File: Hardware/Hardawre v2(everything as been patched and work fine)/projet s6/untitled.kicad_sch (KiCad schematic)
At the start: 28 parts, among them IC1 QMC5883L, J1 USB_C_Receptacle_USB2.0_14P, J2 OLED, Q1 2N7002K, SW1 Boutton 1, SW2 Boutton 2, U4 USBLC6-2SC6

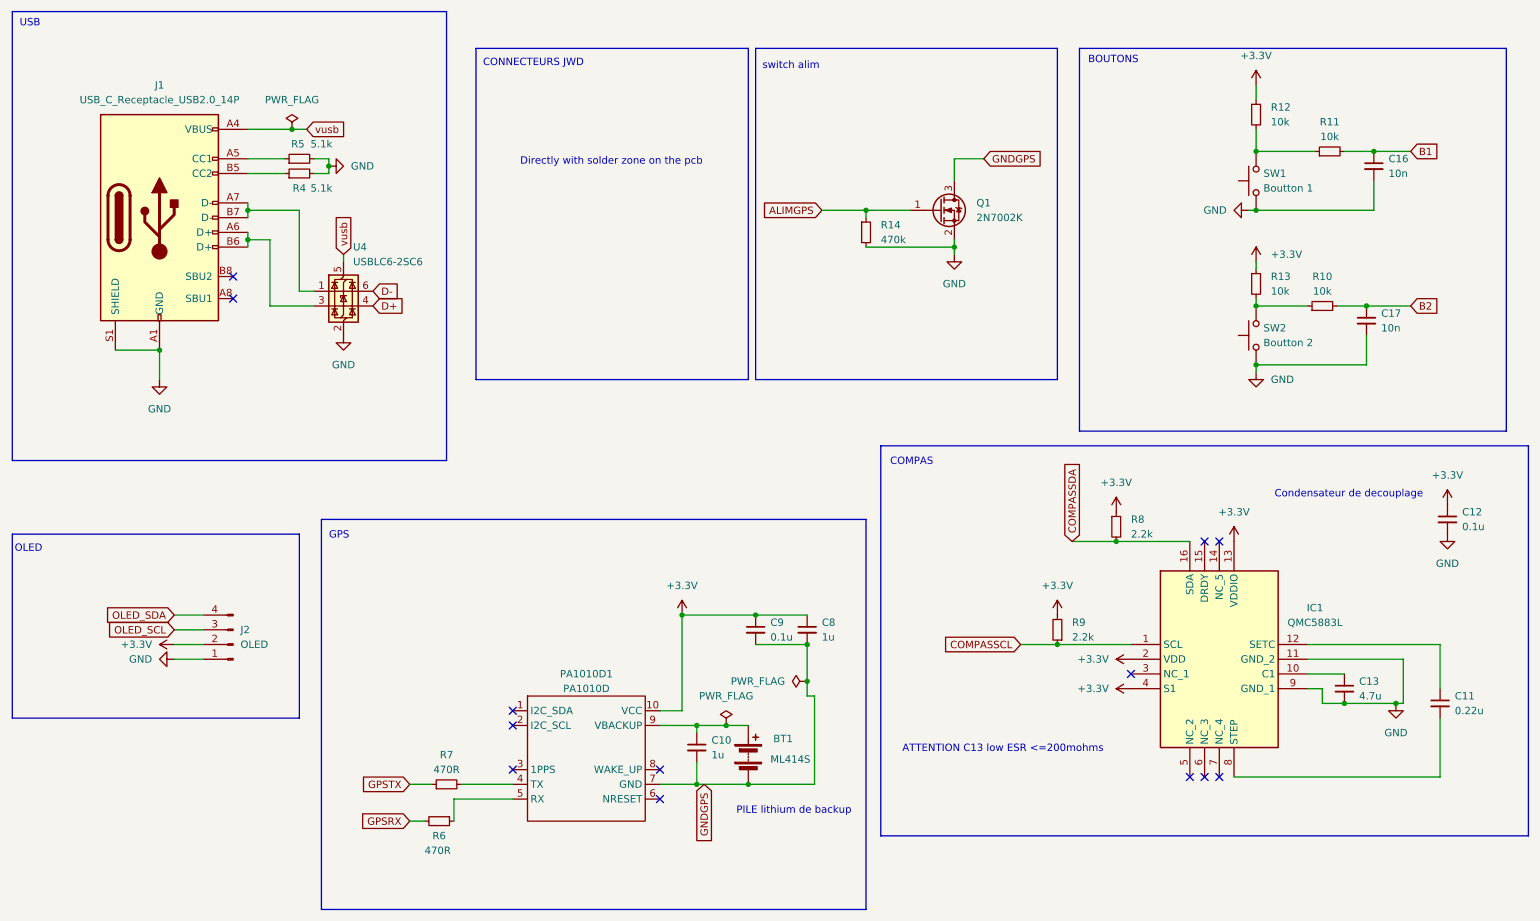
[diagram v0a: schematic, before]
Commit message: gr
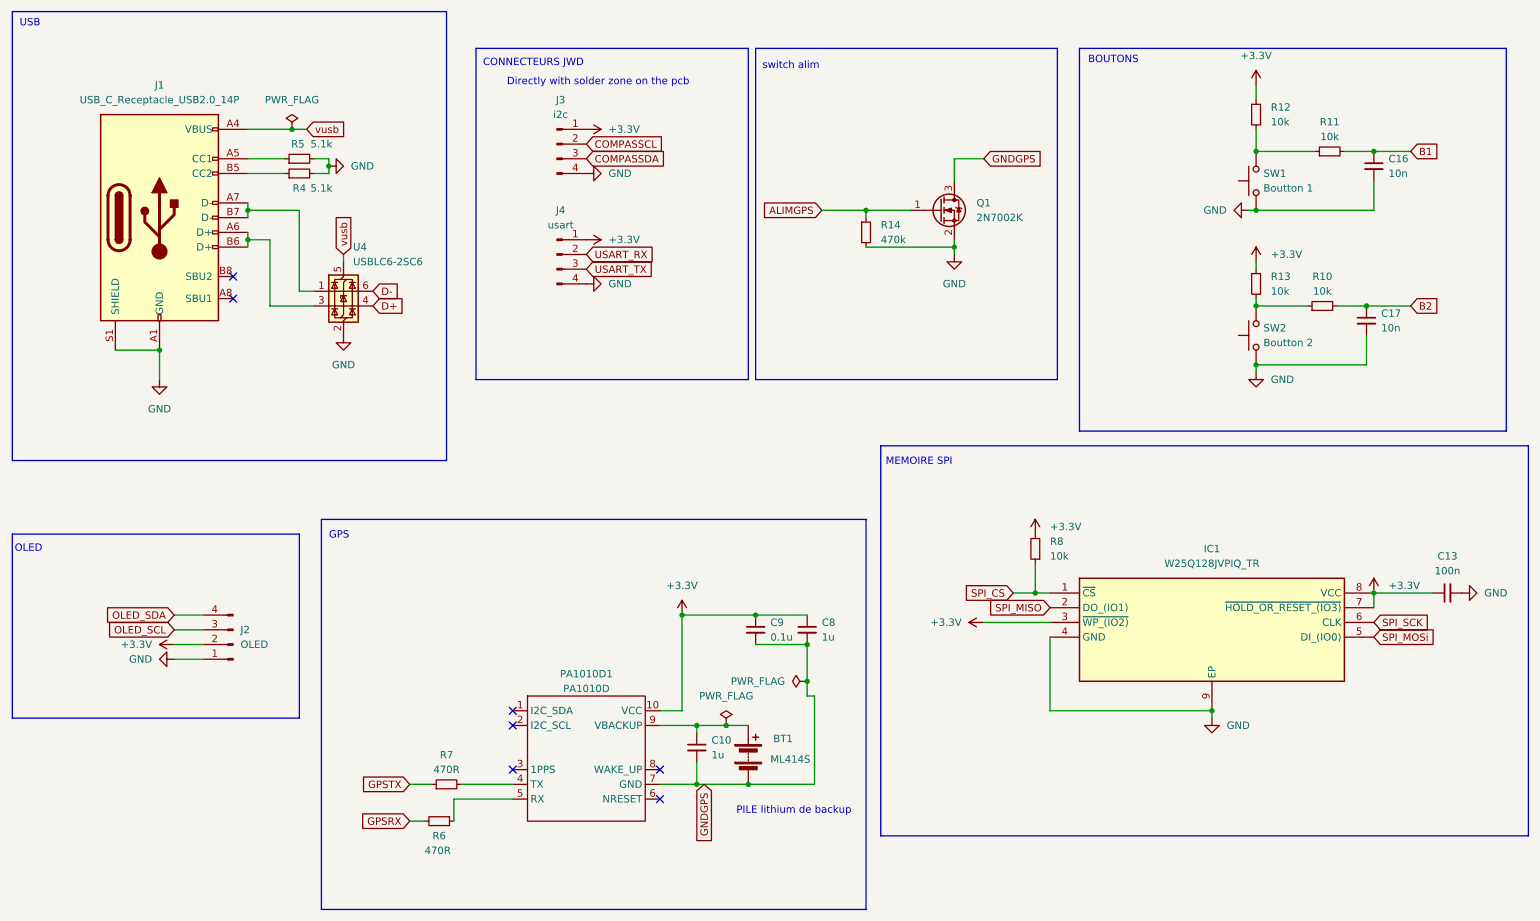
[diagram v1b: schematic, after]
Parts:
- removed C11: 0.22u, Capacitor_SMD:C_0402_1005Metric_Pad0.74x0.62mm_HandSolder, symbol Device:C_Small
- removed C12: 0.1u, Capacitor_SMD:C_0402_1005Metric_Pad0.74x0.62mm_HandSolder, symbol Device:C_Small
- removed IC1: QMC5883L, QMC5883L:QMC5883L, symbol QMC5883L:QMC5883L
- removed R9: 2.2k, Resistor_SMD:R_0402_1005Metric_Pad0.72x0.64mm_HandSolder, symbol Device:R_Small
- added IC1: W25Q128JVPIQ_TR, winbond:SON127P600X500X80-9N-D, symbol winbond:W25Q128JVPIQ_TR
- added J3: i2c, Connector_JST:JST_SH_BM04B-SRSS-TB_1x04-1MP_P1.00mm_Vertical, symbol Connector:Conn_01x04_Pin
- added J4: usart, Connector_JST:JST_SH_BM04B-SRSS-TB_1x04-1MP_P1.00mm_Vertical, symbol Connector:Conn_01x04_Pin
- BT1: footprint MS414:MS421R-IV03E -> MS421R-IV03E:MS421R-IV03E
- C13: value 4.7u -> 100n; footprint Capacitor_SMD:C_0603_1608Metric_Pad1.08x0.95mm_HandSolder -> Capacitor_SMD:C_0402_1005Metric_Pad0.74x0.62mm_HandSolder
- J1: footprint USB4110_USBC_SMT:USB4110_USBC_SMT -> USBC-WURTH:USBC-WURTH
- R8: value 2.2k -> 10k
- SW1, SW2: footprint SW_PTS840:SW_PTS840 -> PTS840:SW_PTS840
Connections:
- net +3.3V: now also C13.1, R8.2, IC1.3 (~{WP_(IO2)}), IC1.7 (~{HOLD_OR_RESET_(IO3)}), IC1.8 (VCC), J3.1 (Pin_1), J4.1 (Pin_1); no longer R8.1
- net COMPASSCL: now also J3.2 (Pin_2)
- net COMPASSDA: now also J3.3 (Pin_3); no longer R8.2
- net GND: now also IC1.4 (GND), IC1.9 (EP), J3.4 (Pin_4), J4.4 (Pin_4)
- new net SPI_CS: IC1.1 (~{CS}), R8.1
- new net SPI_MISO: IC1.2 (DO_(IO1))
- new net SPI_MOSi: IC1.5 (DI_(IO0))
- new net SPI_SCK: IC1.6 (CLK)
- new net USART_RX: J4.2 (Pin_2)
- new net USART_TX: J4.3 (Pin_3)
- no-connect marks 13 -> 7
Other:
- note added: "MEMOIRE SPI"
- note removed: "ATTENTION C13 low ESR <=200mohms"
- note removed: "COMPAS"
- note removed: "Condensateur de decouplage"

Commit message: hardware v3
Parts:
- BT1: footprint MS421R-IV03E:MS421R-IV03E -> MS414:MS421R-IV03E
- J1: footprint USBC-WURTH:USBC-WURTH -> vraieusbwurth:USBC-WURTH
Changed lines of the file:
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@@
 			)
 		)
-		(property "Footprint" "MS421R-IV03E:MS421R-IV03E"
+		(property "Footprint" "MS414:MS421R-IV03E"
 			(at 143.51 143.256 90)
 			(effects
@@
 			)
 		)
-		(property "Footprint" "USBC-WURTH:USBC-WURTH"
+		(property "Footprint" "vraieusbwurth:USBC-WURTH"
 			(at 45.72 52.07 0)
 			(effects
